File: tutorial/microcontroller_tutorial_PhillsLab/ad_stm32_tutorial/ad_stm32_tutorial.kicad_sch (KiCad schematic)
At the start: 0 parts

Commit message: VIDEO #3 :: finished schematic
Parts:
- added C1, C2: 4u7, Capacitor_SMD:C_0805_2012Metric, symbol Device:C
- added C3: 22p, Capacitor_SMD:C_0603_1608Metric, symbol Device:C
- added L1: NRH2412T100MNGH, Inductor_SMD:NRH2412T2R2MNGH, symbol Device:NRH2412T100MNGH
- added R1, R2: 887k, Resistor_SMD:R_0603_1608Metric, symbol Device:R
- added U1: ~, Package_TO_SOT_SMD:SOT-23-6, symbol Regulator_Switching:LTC3405
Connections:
- new net: C3.1, R1.1, R2.1, U1.5 (VFB)
- new net: L1.1, U1.3 (SW)
- new net +3V3: C2.1, C3.2, L1.2, R1.2
- new net +5V: C1.1, U1.1 (RUN), U1.4 (VIN)
- new net GND: C1.2, C2.2, R2.2, U1.2 (GND), U1.6 (MODE)

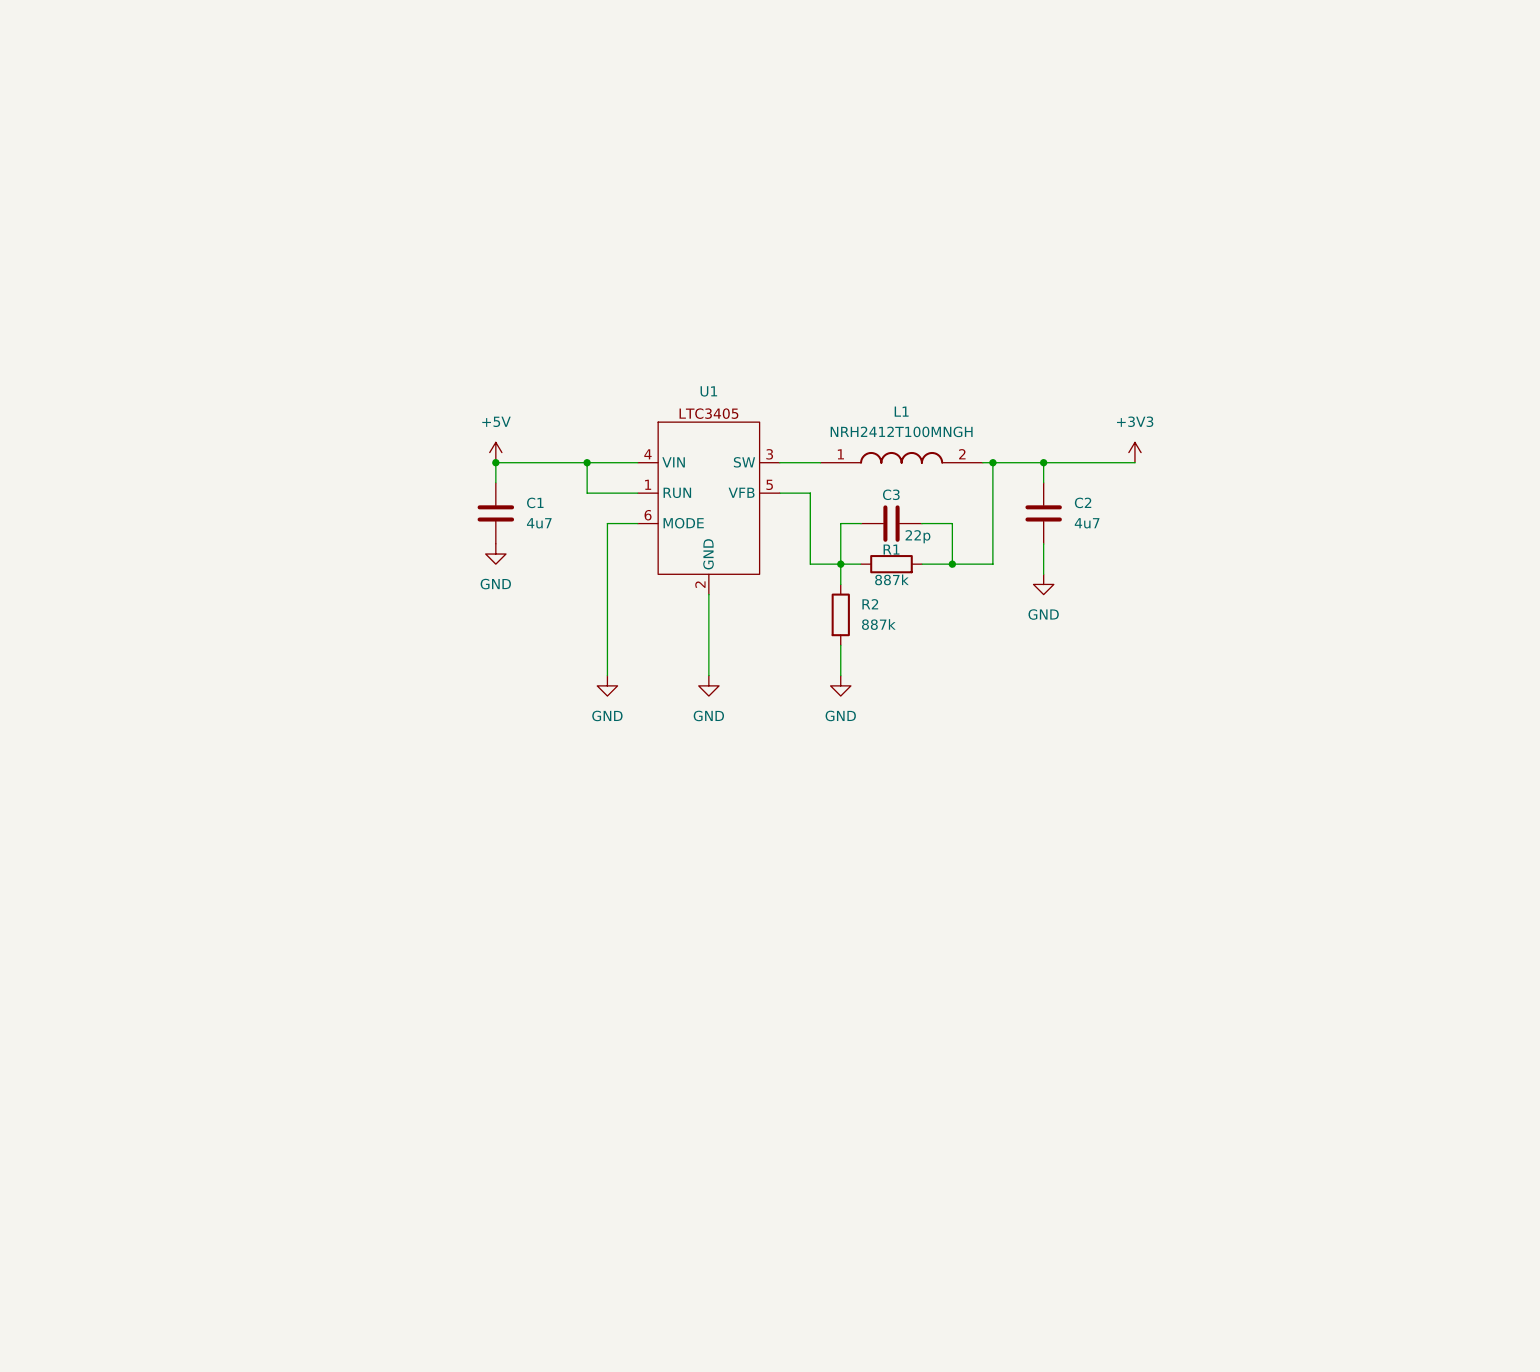
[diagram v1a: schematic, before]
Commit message: VIDEO #3 :: Added USB-C connector
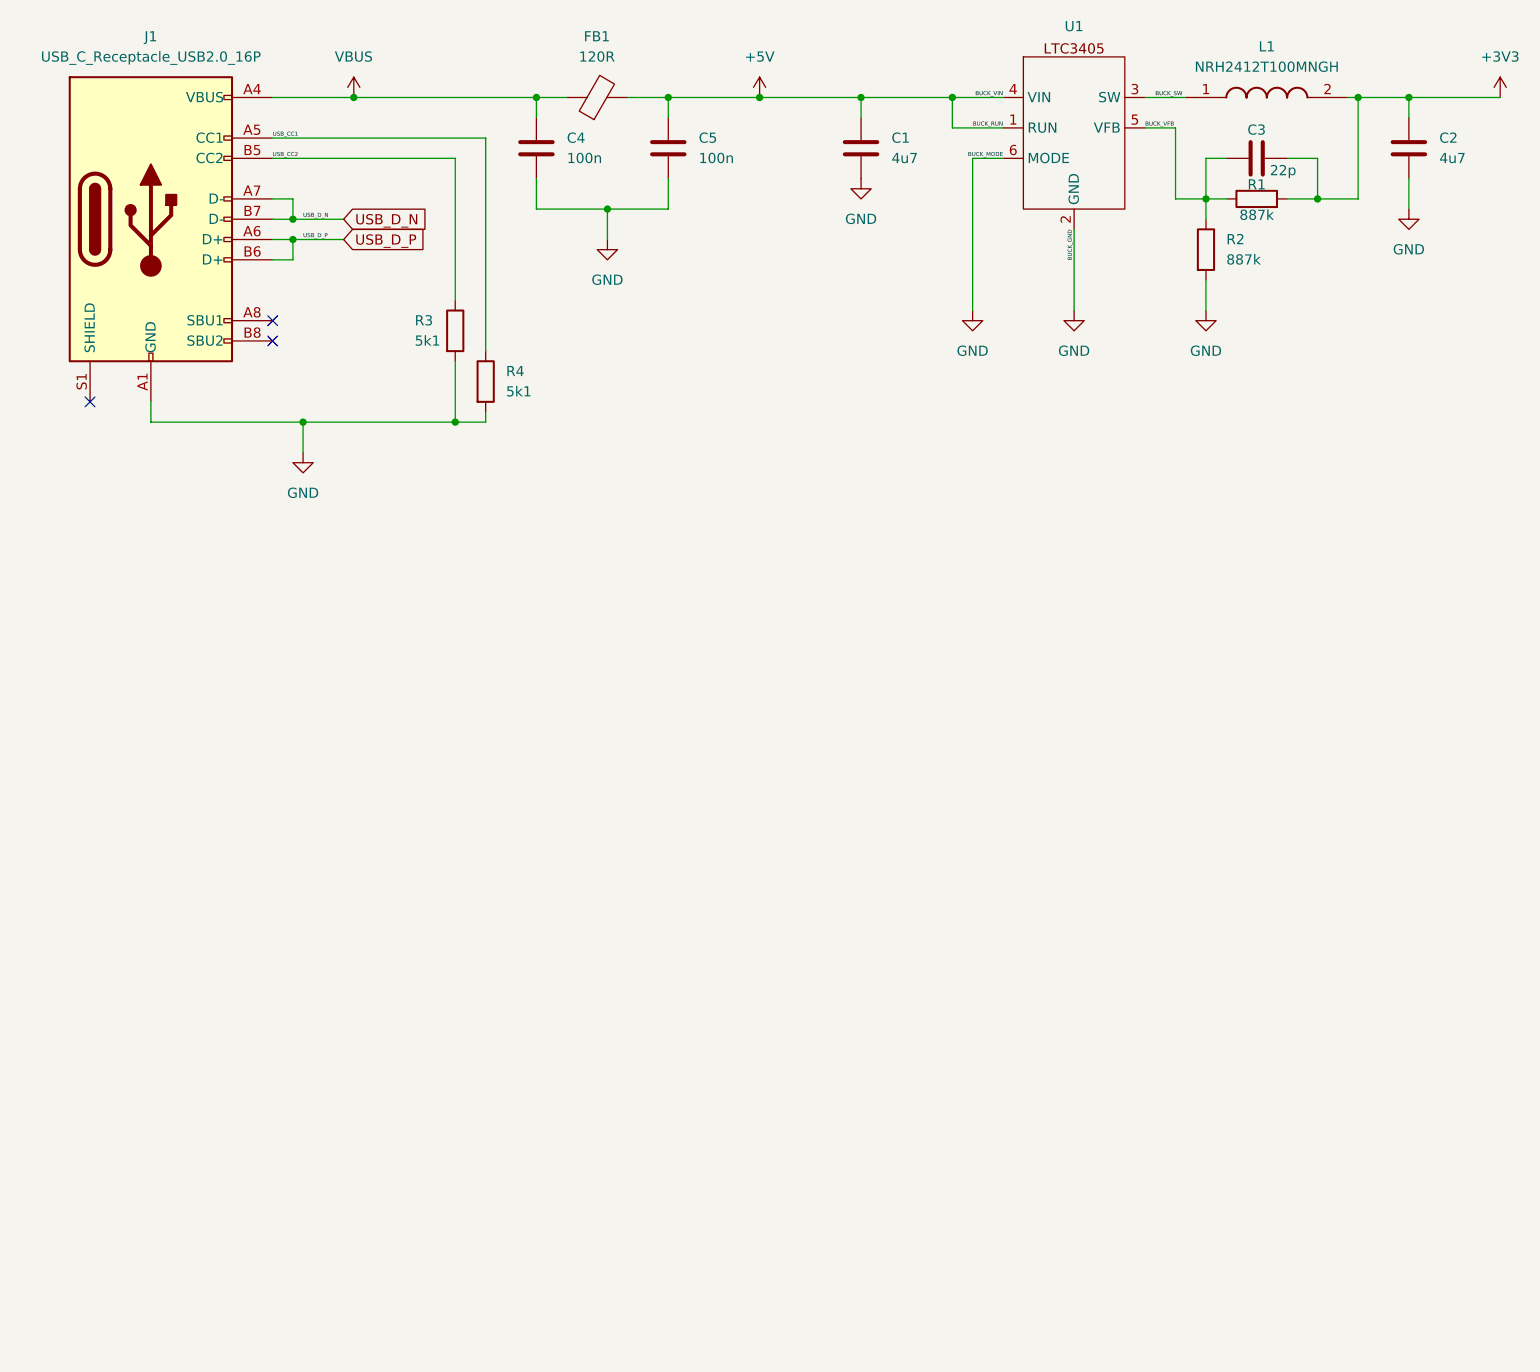
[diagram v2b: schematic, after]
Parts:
- added C4, C5: 100n, Capacitor_SMD:C_0603_1608Metric, symbol Device:C
- added FB1: 120R, Inductor_SMD:L_6.3x6.3_H3, symbol Device:FerriteBead
- added J1: USB_C_Receptacle_USB2.0_16P, Connector_USB:USB_C_Receptacle_GCT_USB4105-xx-A_16P_TopMnt_Horizontal, symbol Connector:USB_C_Receptacle_USB2.0_16P
- added R3, R4: 5k1, Resistor_SMD:R_0603_1608Metric, symbol Device:R
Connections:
- net +5V: now also C5.1, FB1.2
- net GND: now also C4.2, C5.2, J1.A1 (GND), J1.A12 (GND), J1.B1 (GND), J1.B12 (GND), R3.2, R4.2
- net BUCK_VFB: now reaches C3.1, R1.1, R2.1, U1.5 (VFB)
- net BUCK_SW: now reaches L1.1, U1.3 (SW)
- new net USB_CC1: J1.A5 (CC1), R4.1
- new net USB_CC2: J1.B5 (CC2), R3.1
- new net USB_D_N: J1.A7 (D-), J1.B7 (D-)
- new net USB_D_P: J1.A6 (D+), J1.B6 (D+)
- new net VBUS: C4.1, FB1.1, J1.A4 (VBUS), J1.A9 (VBUS), J1.B4 (VBUS), J1.B9 (VBUS)
- no-connect marks 0 -> 3
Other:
- moved on the sheet: C1, C2, C3, L1, R1, R2, U1

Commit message: Finished Video 4 of Phil's Lab Microcontroller-Based Hardware Design tutorial
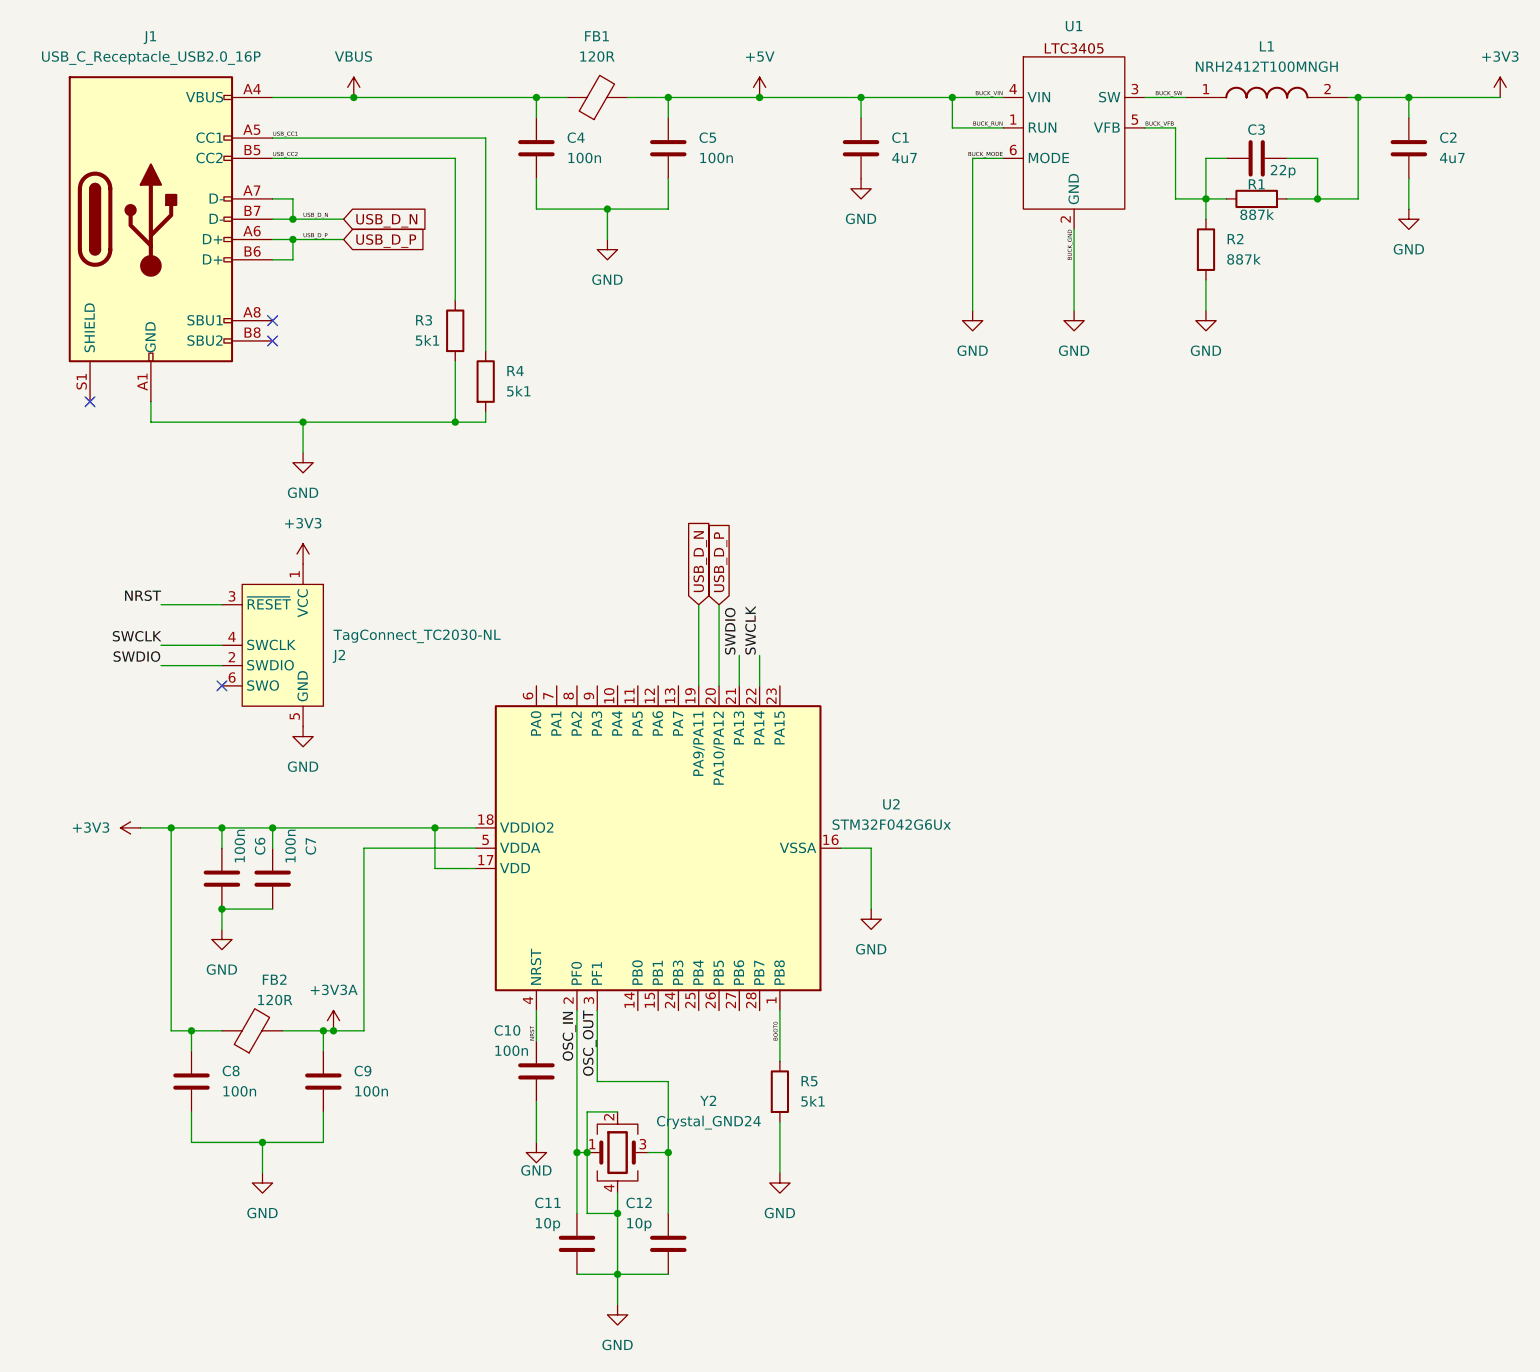
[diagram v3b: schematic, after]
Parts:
- added C10, C6, C7, C8, C9: 100n, Capacitor_SMD:C_0603_1608Metric, symbol Device:C
- added C11, C12: 10p, Capacitor_SMD:C_0603_1608Metric, symbol Device:C
- added FB2: 120R, Inductor_SMD:L_6.3x6.3_H3, symbol Device:FerriteBead
- added J2: TagConnect_TC2030-NL, Connector:Tag-Connect_TC2030-IDC-NL_2x03_P1.27mm_Vertical, symbol Connector:Conn_ARM_SWD_TagConnect_TC2030-NL
- added R5: 5k1, Resistor_SMD:R_0603_1608Metric, symbol Device:R
- added U2: STM32F042G6Ux, Package_DFN_QFN:QFN-28_4x4mm_P0.5mm, symbol MCU_ST_STM32F0:STM32F042G6Ux
- added Y2: Crystal_GND24, symbol Device:Crystal_GND24
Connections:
- net +3V3: now also C6.2, C7.2, C8.1, FB2.1, J2.1 (VCC), U2.17 (VDD), U2.18 (VDDIO2)
- net GND: now also C10.2, C11.1, C11.2, C12.2, C6.1, C7.1, C8.2, C9.2, J2.5 (GND), R5.2, U2.16 (VSSA), U2.2 (PF0), Y2.1, Y2.2, Y2.4
- net USB_D_N: now also U2.19 (PA9/PA11)
- net USB_D_P: now also U2.20 (PA10/PA12)
- new net +3V3A: C9.1, FB2.2, U2.5 (VDDA)
- new net BOOT0: R5.1, U2.1 (PB8)
- new net NRST: C10.1, J2.3 (~{RESET}), U2.4 (NRST)
- new net OSC_OUT: C12.1, U2.3 (PF1), Y2.3
- new net SWCLK: J2.4 (SWCLK), U2.22 (PA14)
- new net SWDIO: J2.2 (SWDIO), U2.21 (PA13)
- no-connect marks 3 -> 4
